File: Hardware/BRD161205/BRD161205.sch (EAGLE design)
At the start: 15 parts, among them CN1 MOLEX 4455, U1 TPS73101, U2 PL133-37, U3 74VHC04, X1 10MHz

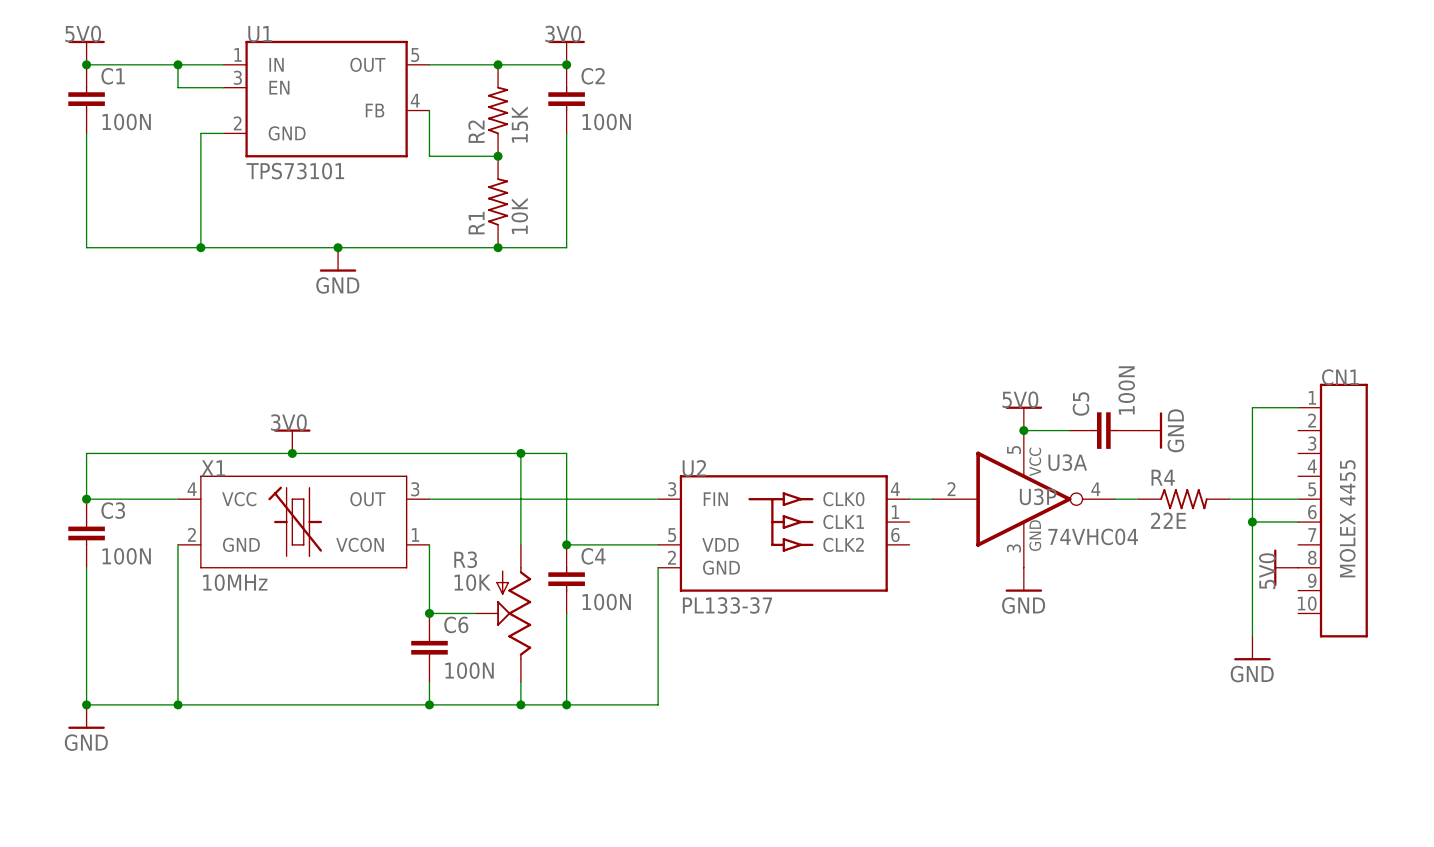
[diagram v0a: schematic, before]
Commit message: BRD161205 R0
Signed-off-by: Christoph Tack <prog.send@gmail.com>
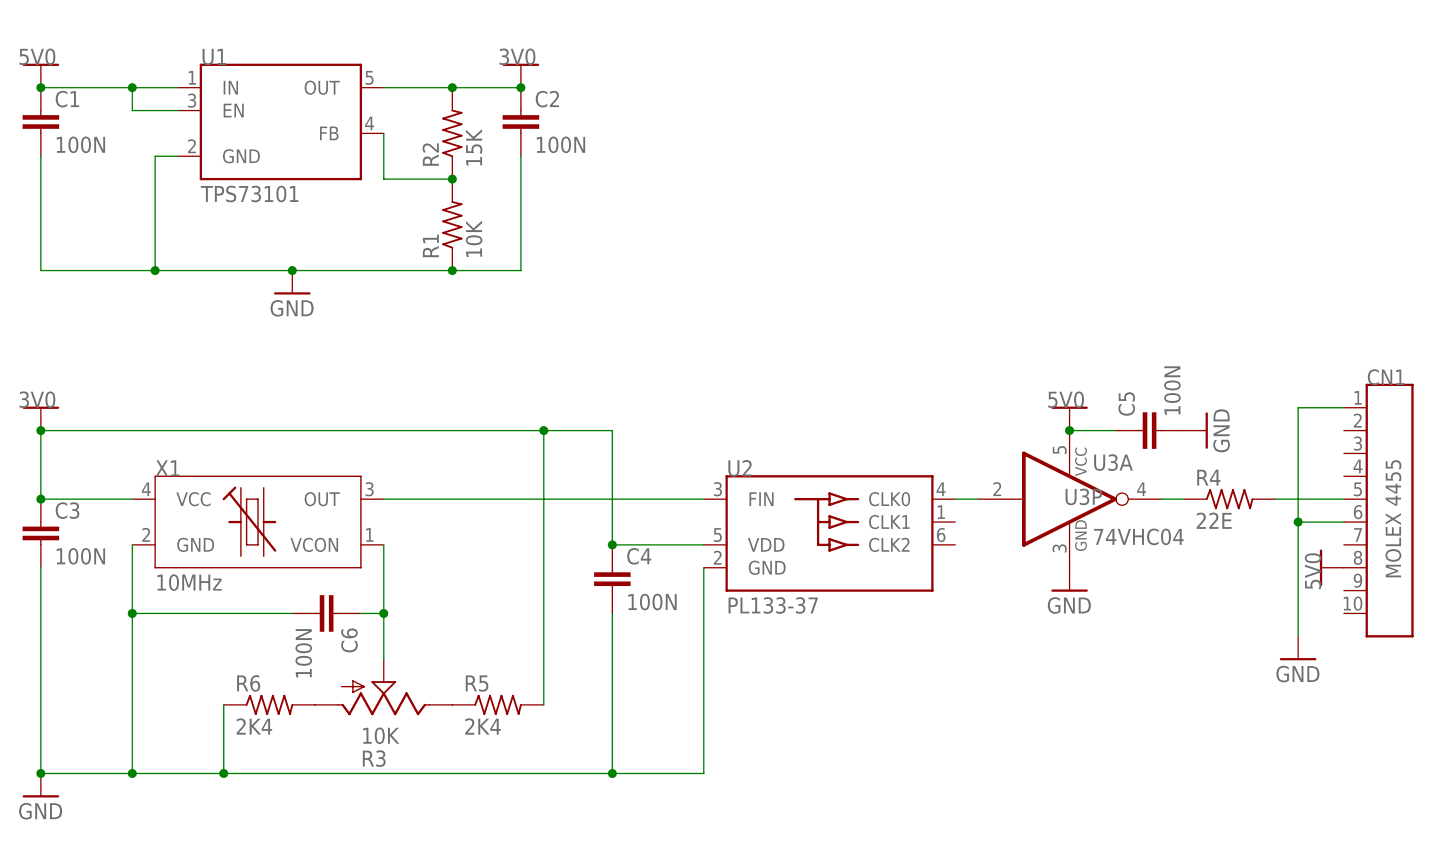
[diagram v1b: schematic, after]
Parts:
- added R5, R6: 2K4, lieBtrau:RE_2K4_1206
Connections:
- new net N$7: R3.3, R5.1
- new net N$8: R3.1, R6.2
- net 3V0: now also R5.2; no longer R3.1
- net GND: now also R6.1; no longer R3.3
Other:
- moved on the sheet: C1, C2, C3, C4, C5, C6, CN1, R1, R2, R3, R4, U1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
